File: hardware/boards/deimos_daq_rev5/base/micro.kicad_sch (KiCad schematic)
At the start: 89 parts, among them IC1 STM32H743ZIT6, J4 Conn_02x07_Odd_Even, Y1 SiT1602BI-21-33S-48.000000

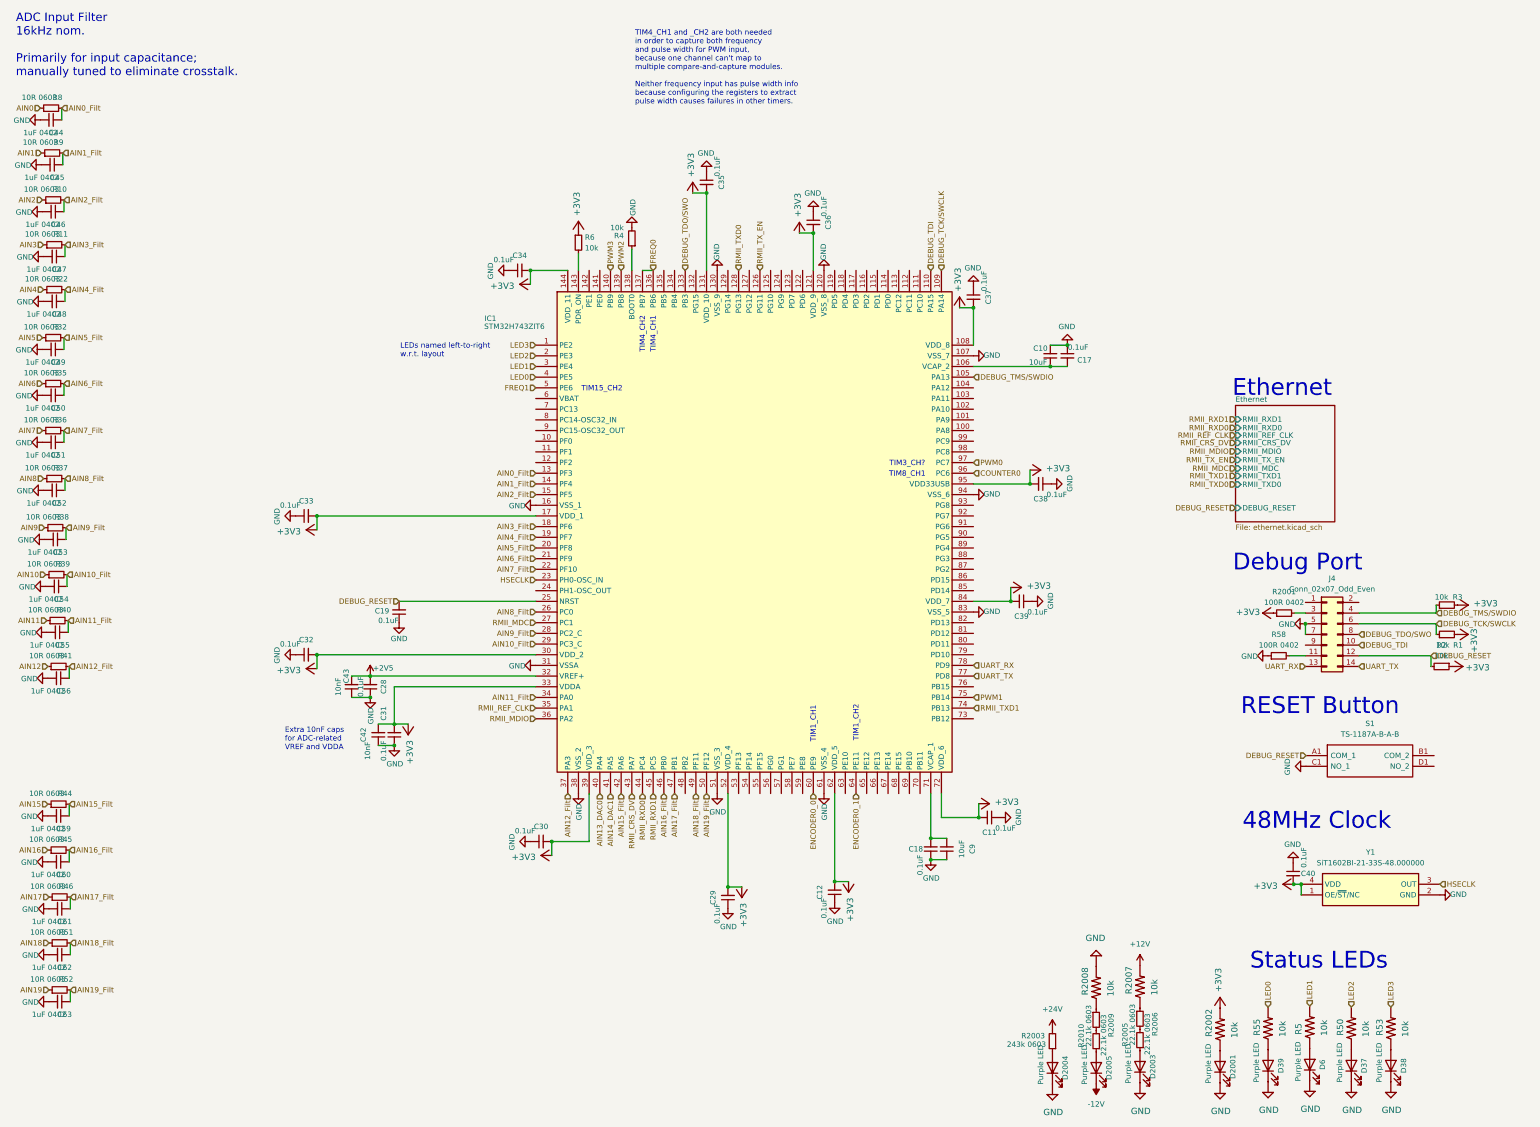
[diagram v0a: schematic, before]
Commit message: restore rev5 and make this rev rev6
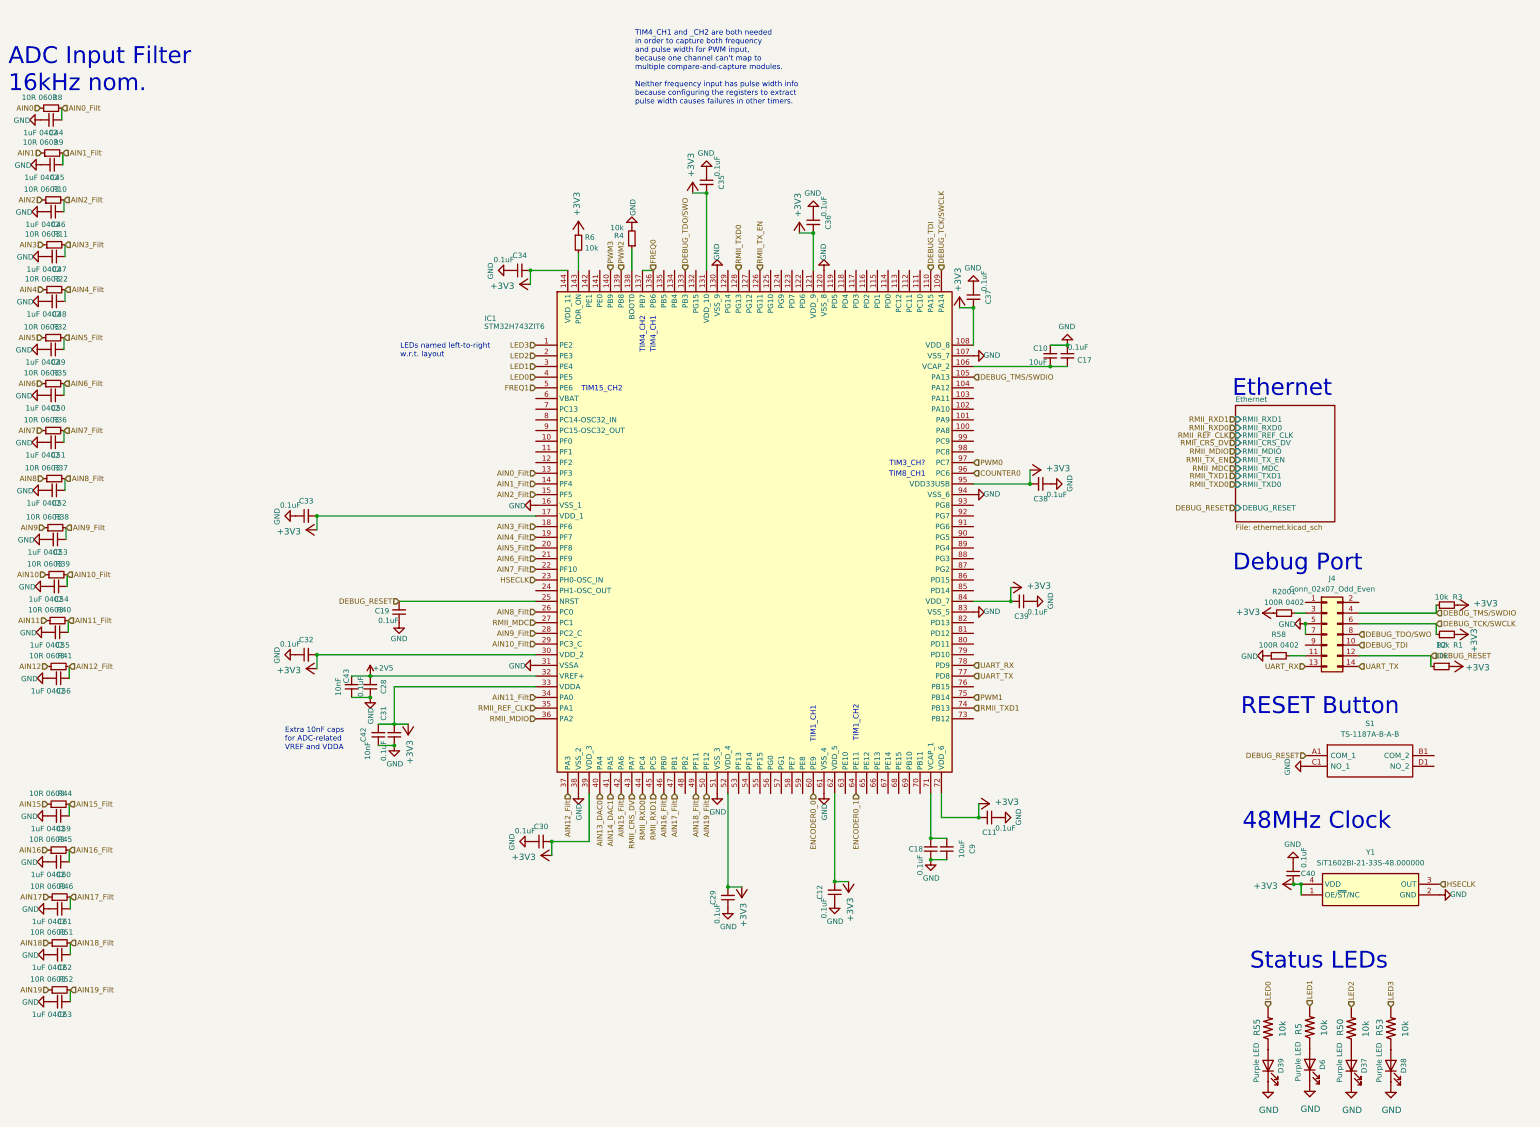
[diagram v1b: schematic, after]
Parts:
- removed D2001, D2003, D2004, D2005: Purple LED, LED_SMD:LED_0603_1608Metric, symbol Device:LED
- removed R2002, R2007, R2008: 10k, Resistor_SMD:R_0402_1005Metric, symbol EK-TM4C1294XL_REV_D-eagle-import:R-US_R0402
- removed R2003: 243k 0603, Resistor_SMD:R_0603_1608Metric, symbol Device:R_Small
- removed R2005, R2006, R2009, R2010: 22.1k 0603, Resistor_SMD:R_0603_1608Metric, symbol Device:R_Small
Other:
- note added: "ADC Input Filter 16kHz nom."
- note removed: "ADC Input Filter 16kHz nom. Primarily for input capacitance; manually tuned to eliminate crosstalk."

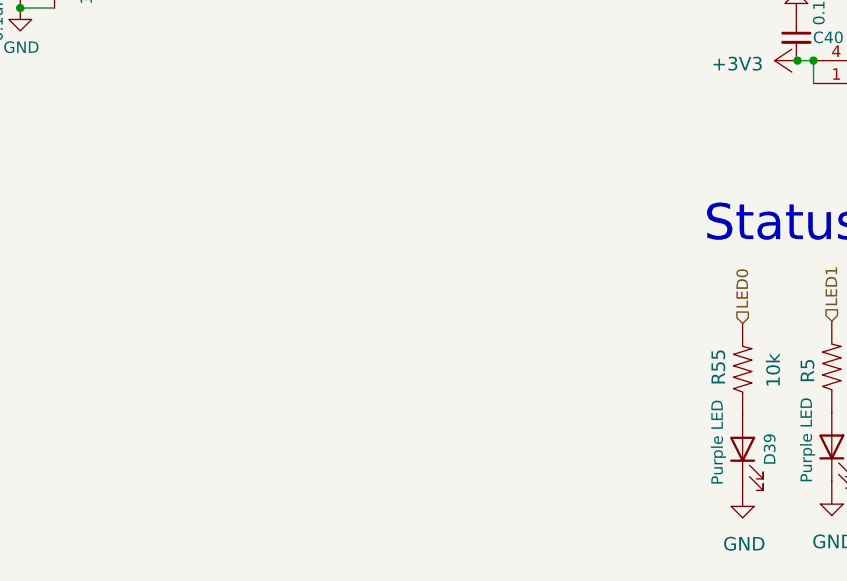
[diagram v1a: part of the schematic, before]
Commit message: add more status leds
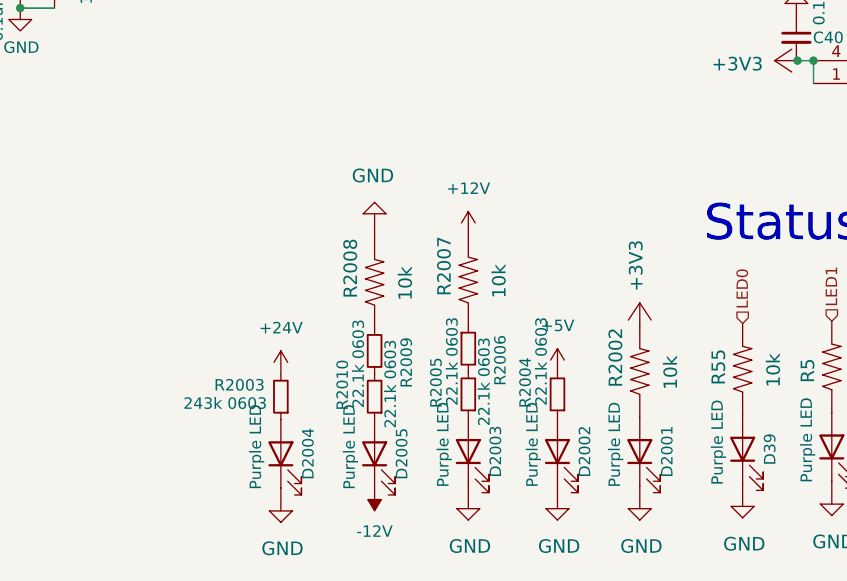
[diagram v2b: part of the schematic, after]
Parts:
- added D2001, D2002, D2003, D2004, D2005: Purple LED, LED_SMD:LED_0603_1608Metric, symbol Device:LED
- added R2002, R2007, R2008: 10k, Resistor_SMD:R_0402_1005Metric, symbol EK-TM4C1294XL_REV_D-eagle-import:R-US_R0402
- added R2003: 243k 0603, Resistor_SMD:R_0603_1608Metric, symbol Device:R_Small
- added R2004, R2005, R2006, R2009, R2010: 22.1k 0603, Resistor_SMD:R_0603_1608Metric, symbol Device:R_Small
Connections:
- net +3V3: now also R2002.2
- net GND: now also D2001.1 (K), D2002.1 (K), D2003.1 (K), D2004.1 (K), R2008.2
- new net: D2003.2 (A), R2005.1
- new net: D2004.2 (A), R2003.1
- new net: R2005.2, R2006.2
- new net: D2001.2 (A), R2002.1
- new net: D2005.2 (A), R2010.1
- new net: R2008.1, R2009.1
- new net: R2009.2, R2010.2
- new net: D2002.2 (A), R2004.1
- new net: R2006.1, R2007.1
- new net +12V: R2007.2
- new net +24V: R2003.2
- new net +5V: R2004.2
- new net -12V: D2005.1 (K)
